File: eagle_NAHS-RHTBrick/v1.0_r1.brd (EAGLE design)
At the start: 45.5 x 70.3 mm, 47 parts, among them IC1 ESP12S, IC2 ATTINY212-SSNR, IC3 TP4056, IC4 DW01A, IC5 HDC1080, J1 10118194-0001LF, J2 BRICK-INTERF-V3_B-SIDE, Q1 8205A, T1 PINHD_1X03_R_1, T2 PINHD_1X03_R_1, T3 PINHD_1X03_R_1

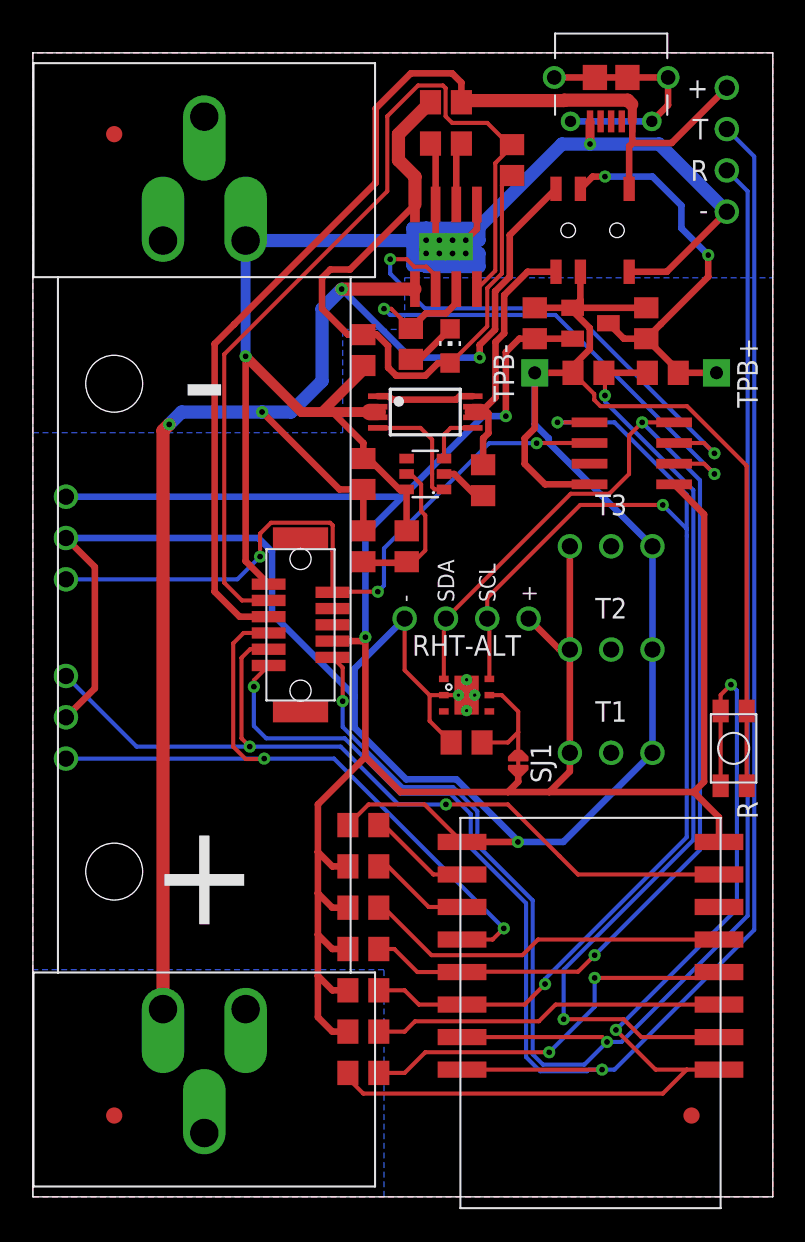
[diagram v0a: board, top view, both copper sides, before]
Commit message: saving
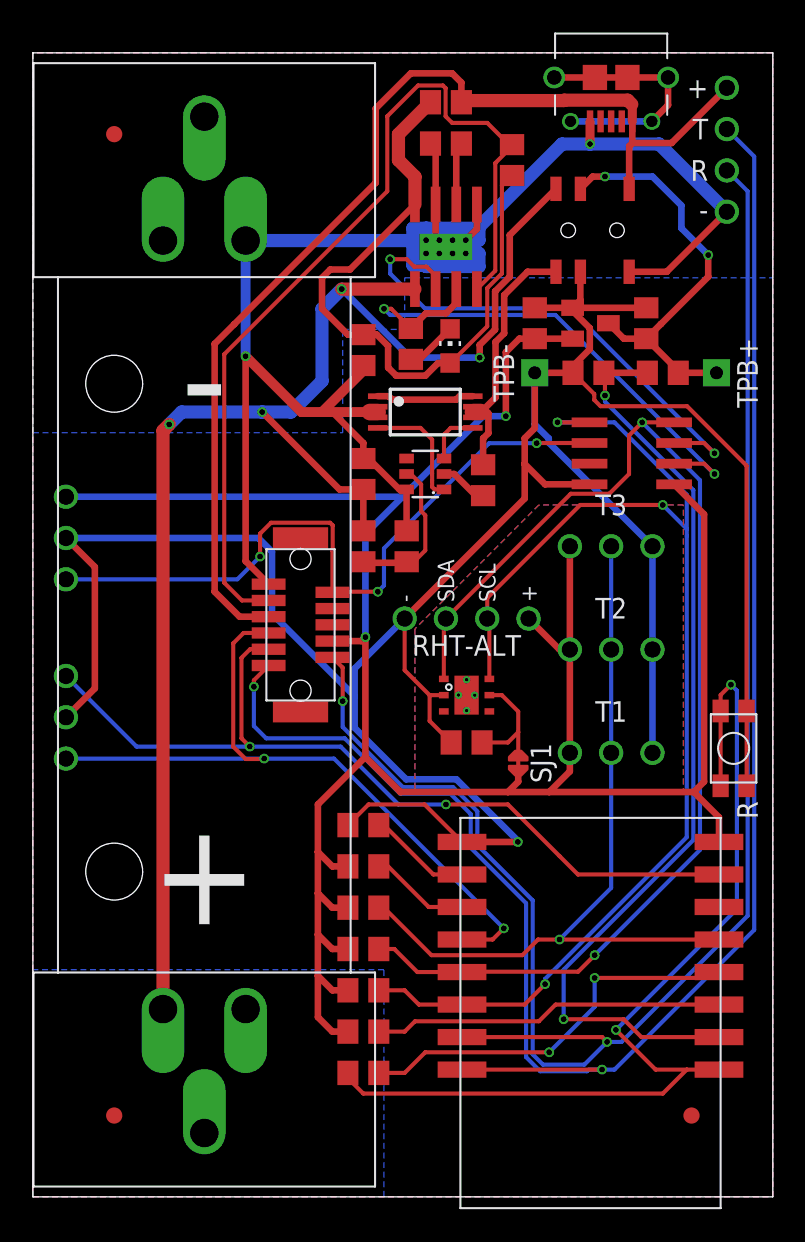
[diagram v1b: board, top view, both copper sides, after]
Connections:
- net GND: no longer IC5.7, IC5.7.1, IC5.7.2, IC5.7.3, IC5.7.4
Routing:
- net 1WIRE: track 22.5 -> 48.0 mm, vias 0 -> 1
- net GND: track 176.7 -> 177.8 mm
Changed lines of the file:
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@@
 <setting verticaltext="up"/>
 </settings>
-<grid distance="25" unitdist="mil" unit="mil" style="lines" multiple="1" display="yes" altdistance="5" altunitdist="mil" altunit="mil"/>
+<grid distance="25" unitdist="mil" unit="mm" style="lines" multiple="1" display="yes" altdistance="5" altunitdist="mil" altunit="mil"/>
 <layers>
 <layer number="1" name="Top" color="4" fill="1" visible="yes" active="yes"/>
@@
 </class>
 </classes>
-<designrules name="JLCPCB">
+<designrules name="JLCPCB *">
 <description language="de">&lt;b&gt;EAGLE Design Rules&lt;/b&gt;
 &lt;p&gt;
@@
 <param name="rvMicroViaOuter" value="0.25"/>
 <param name="rvMicroViaInner" value="0.25"/>
-<param name="rlMinPadTop" value="10mil"/>
+<param name="rlMinPadTop" value="0.13mm"/>
 <param name="rlMaxPadTop" value="20mil"/>
 <param name="rlMinPadInner" value="10mil"/>
 <param name="rlMaxPadInner" value="20mil"/>
-<param name="rlMinPadBottom" value="10mil"/>
+<param name="rlMinPadBottom" value="0.13mm"/>
 <param name="rlMaxPadBottom" value="20mil"/>
-<param name="rlMinViaOuter" value="8mil"/>
+<param name="rlMinViaOuter" value="0.13mm"/>
 <param name="rlMaxViaOuter" value="20mil"/>
 <param name="rlMinViaInner" value="8mil"/>
@@
 <wire x1="30.861" y1="47.26575" x2="30.861" y2="50.673" width="0.4064" layer="1"/>
 <wire x1="30.243325" y1="46.648075" x2="30.861" y2="47.26575" width="0.4064" layer="1"/>
-<wire x1="30.243325" y1="45.067675" x2="30.243325" y2="46.648075" width="0.4064" layer="1"/>
+<wire x1="30.243325" y1="45.067675" x2="30.243325" y2="45.085" width="0.4064" layer="1"/>
+<wire x1="30.243325" y1="45.085" x2="30.243325" y2="46.648075" width="0.4064" layer="1"/>
 <wire x1="31.496" y1="43.815" x2="30.243325" y2="45.067675" width="0.4064" layer="1"/>
 <wire x1="40.23173125" y1="48.6184" x2="43.88613125" y2="44.964" width="0.254" layer="1"/>
@@
 <wire x1="43.88613125" y1="44.964" x2="43.88613125" y2="29.877" width="0.254" layer="1"/>
 <contactref element="IC5" pad="2"/>
-<contactref element="IC5" pad="7.1"/>
-<contactref element="IC5" pad="7"/>
-<contactref element="IC5" pad="7.3"/>
-<contactref element="IC5" pad="7.4"/>
-<contactref element="IC5" pad="7.2"/>
 <contactref element="T1" pad="3"/>
 <contactref element="T2" pad="3"/>
@@
 <wire x1="38.1" y1="40.005" x2="38.1" y2="33.655" width="0.4064" layer="16"/>
 <wire x1="38.1" y1="27.305" x2="38.1" y2="33.655" width="0.4064" layer="16"/>
-<wire x1="38.1" y1="27.305" x2="32.618" y2="21.823" width="0.4064" layer="16"/>
-<wire x1="32.618" y1="21.823" x2="29.824" y2="21.823" width="0.4064" layer="16"/>
 <contactref element="RHT-ALT" pad="1"/>
 <wire x1="19.7838" y1="30.78395" x2="19.7838" y2="32.4838" width="0.4064" layer="16"/>
@@
 <wire x1="22.86" y1="32.385" x2="22.86" y2="35.56" width="0.254" layer="1"/>
 <wire x1="24.395" y1="30.85" x2="22.86" y2="32.385" width="0.254" layer="1"/>
-<wire x1="25.27" y1="30.85" x2="26.17" y2="30.85" width="0.254" layer="1"/>
 <contactref element="C6" pad="2"/>
 <wire x1="25.72" y1="27.94" x2="24.395" y2="29.265" width="0.254" layer="1"/>
 <wire x1="24.395" y1="29.265" x2="24.395" y2="30.85" width="0.254" layer="1"/>
-<wire x1="27.17" y1="30.85" x2="26.67" y2="30.85" width="0" layer="19" extent="1-1"/>
-<wire x1="26.17" y1="30.85" x2="26.67" y2="30.85" width="0" layer="19" extent="1-1"/>
-<wire x1="26.67" y1="31.8" x2="26.67" y2="30.85" width="0" layer="19" extent="1-1"/>
-<wire x1="26.67" y1="29.9" x2="26.67" y2="30.85" width="0" layer="19" extent="1-1"/>
+<wire x1="30.243325" y1="45.067675" x2="30.243325" y2="42.943325" width="0.4064" layer="1"/>
+<wire x1="30.243325" y1="42.943325" x2="22.86" y2="35.56" width="0.4064" layer="1"/>
+<polygon width="0.1524" layer="1" pour="cutout">
+<vertex x="23.495" y="24.765"/>
+<vertex x="40.005" y="24.765"/>
+<vertex x="40.005" y="42.545"/>
+<vertex x="31.115" y="42.545"/>
+<vertex x="23.495" y="34.925"/>
+</polygon>
+<polygon width="0.1524" layer="16" pour="cutout" rank="2">
+<vertex x="23.495" y="34.925"/>
+<vertex x="23.495" y="24.765"/>
+<vertex x="40.005" y="24.765"/>
+<vertex x="40.005" y="42.545"/>
+<vertex x="31.115" y="42.545"/>
+</polygon>
 </signal>
 <signal name="SEL+">
@@
 <contactref element="IC1" pad="GPIO14"/>
 <wire x1="21.27" y1="17.78" x2="21.59" y2="17.78" width="0.254" layer="1"/>
-<wire x1="31.063" y1="15.823" x2="42.19" y2="15.823" width="0.254" layer="1"/>
+<wire x1="31.063" y1="15.823" x2="32.385" y2="15.823" width="0.254" layer="1"/>
+<wire x1="32.385" y1="15.823" x2="42.19" y2="15.823" width="0.254" layer="1"/>
 <wire x1="21.59" y1="17.78" x2="24.511" y2="14.859" width="0.254" layer="1"/>
 <wire x1="24.511" y1="14.859" x2="30.099" y2="14.859" width="0.254" layer="1"/>
 <wire x1="30.099" y1="14.859" x2="31.063" y2="15.823" width="0.254" layer="1"/>
 <contactref element="T3" pad="2"/>
-<wire x1="35.56" y1="33.655" x2="35.56" y2="40.005" width="0" layer="19" extent="1-1"/>
-<wire x1="35.56" y1="27.305" x2="35.56" y2="33.655" width="0" layer="19" extent="1-1"/>
-<wire x1="42.19" y1="15.823" x2="35.56" y2="27.305" width="0" layer="19" extent="1-1"/>
+<wire x1="35.56" y1="27.305" x2="35.56" y2="18.998" width="0.254" layer="16"/>
+<wire x1="35.56" y1="18.998" x2="32.385" y2="15.823" width="0.254" layer="16"/>
+<via x="32.385" y="15.823" extent="1-16" drill="0.35"/>
+<wire x1="35.56" y1="27.305" x2="35.56" y2="33.655" width="0.254" layer="16"/>
+<wire x1="35.56" y1="33.655" x2="35.56" y2="40.005" width="0.254" layer="16"/>
 </signal>
 <signal name="N$5">
